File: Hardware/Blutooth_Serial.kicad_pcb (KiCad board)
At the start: 2 copper layers, 67.4 x 48.5 mm, 22 parts, among them J2 Conn_01x04_Pin, U2 MAX3232, U3 LM2596S-5

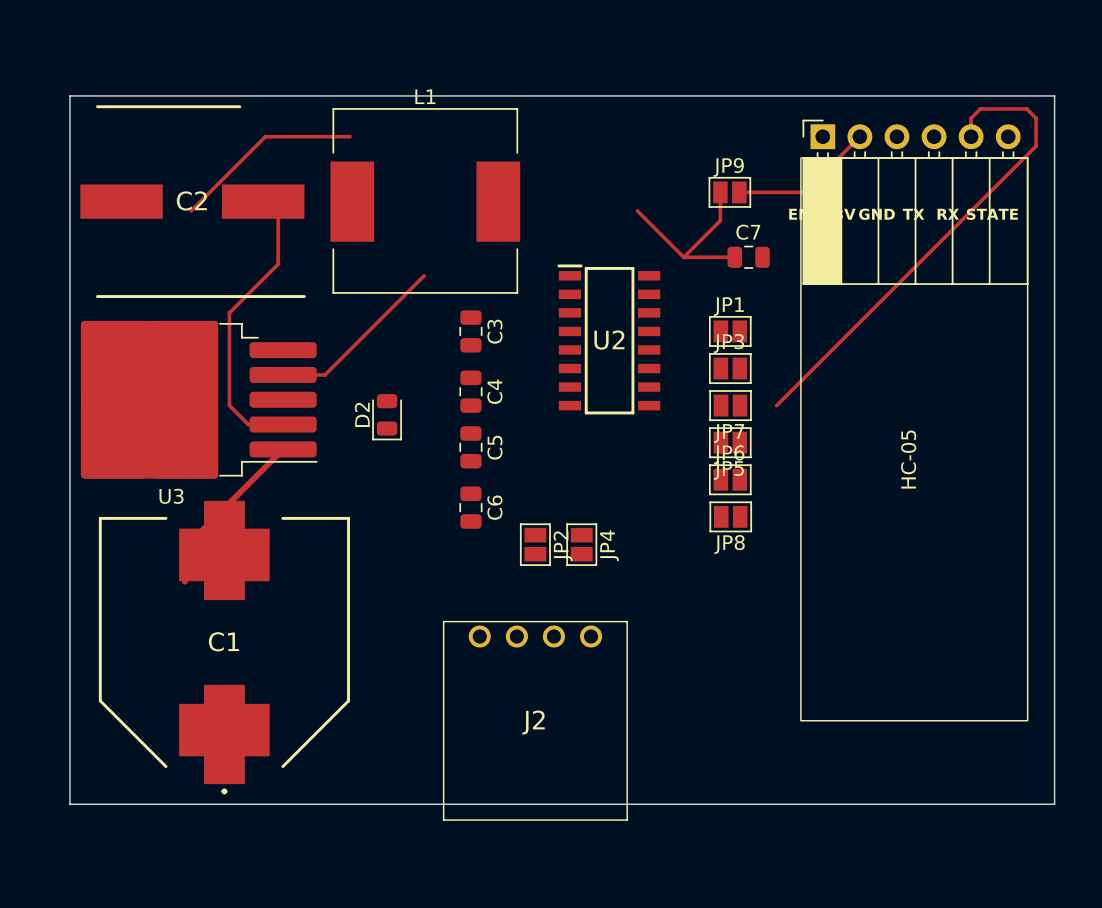
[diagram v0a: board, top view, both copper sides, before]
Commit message: changes
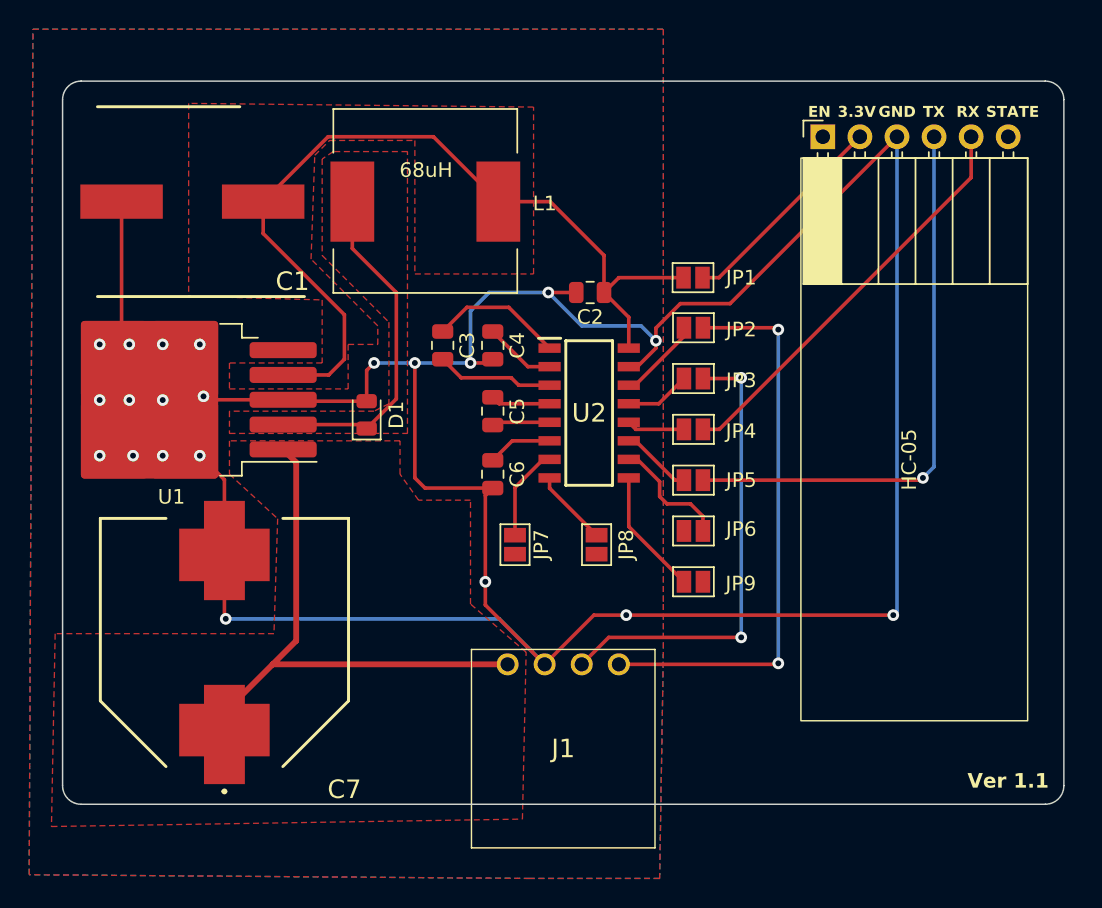
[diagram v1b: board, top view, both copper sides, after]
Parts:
- added G***: LOGO, Library:LOGO, B.Cu at (108.7, 109.0)
- C1: renamed from C2; footprint my_lib:220uF_SMD_CAP -> Library:220uF_SMD_CAP
- C2: renamed from C7; footprint Capacitor_SMD:C_0805_2012Metric -> Library:C_0805_2012Metric
- C3, C4, C5, C6: footprint Capacitor_SMD:C_0805_2012Metric -> Library:C_0805_2012Metric
- C7: renamed from C1; footprint my_lib:470uF_SMD_CAP -> Library:470uF_SMD_CAP
- D1: renamed from D2; footprint Diode_SMD:D_0805_2012Metric -> Library:D_0805_2012Metric
- IC1: footprint my_lib:HC-05 -> Library:HC-05
- J1: renamed from J2; footprint my_lib:male_pin_4 -> Library:male_pin_4
- JP1: renamed from JP9; footprint Jumper:SolderJumper-2_P1.3mm_Open_Pad1.0x1.5mm -> Library:SolderJumper-2_P1.3mm_Open_Pad1.0x1.5mm
- JP2: renamed from JP1; footprint Jumper:SolderJumper-2_P1.3mm_Open_Pad1.0x1.5mm -> Library:SolderJumper-2_P1.3mm_Open_Pad1.0x1.5mm
- JP3, JP5, JP6: footprint Jumper:SolderJumper-2_P1.3mm_Open_Pad1.0x1.5mm -> Library:SolderJumper-2_P1.3mm_Open_Pad1.0x1.5mm
- JP4: renamed from JP7; footprint Jumper:SolderJumper-2_P1.3mm_Open_Pad1.0x1.5mm -> Library:SolderJumper-2_P1.3mm_Open_Pad1.0x1.5mm
- JP7: renamed from JP2; footprint Jumper:SolderJumper-2_P1.3mm_Open_Pad1.0x1.5mm -> Library:SolderJumper-2_P1.3mm_Open_Pad1.0x1.5mm
- JP8: renamed from JP4; footprint Jumper:SolderJumper-2_P1.3mm_Open_Pad1.0x1.5mm -> Library:SolderJumper-2_P1.3mm_Open_Pad1.0x1.5mm
- JP9: renamed from JP8; footprint Jumper:SolderJumper-2_P1.3mm_Open_Pad1.0x1.5mm -> Library:SolderJumper-2_P1.3mm_Open_Pad1.0x1.5mm
- L1: footprint my_lib:L_12x12mm_H6mm -> Library:L_12x12mm_H6mm
- U1: renamed from U3; footprint Package_TO_SOT_SMD:TO-263-5_TabPin3 -> Library:TO-263-5_TabPin3
- U2: footprint my_lib:MAX3232EIDR -> Library:MAX3232EIDR
- moved C2 11.1 mm to (80.6, 76.7), turned to 180 degrees
- moved JP1 6.36 mm to (87.6, 75.7)
- moved U2 5.15 mm to (80.5, 85.0)
- moved JP9 5.13 mm to (87.7, 96.5)
- moved JP6 4.32 mm to (87.7, 93.0)
- moved JP5 3.60 mm to (87.7, 89.6)
- moved C4 3.51 mm to (73.9, 80.3)
- moved JP4 3.02 mm to (87.7, 86.1)
- moved C5 2.89 mm to (73.9, 84.8)
- moved C6 2.73 mm to (73.9, 89.2)
- moved J1 2.69 mm to (78.7, 108.0)
- moved JP3 2.62 mm to (87.7, 82.6)
- moved JP2 2.54 mm to (87.7, 79.1)
- moved C3 2.16 mm to (70.5, 80.3)
- moved D1 1.40 mm to (65.3, 85.1)
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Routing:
- net GND: track 0.00 -> 205.8 mm, vias 0 -> 21
- net Net-(J1-Pin_4): track 0.00 -> 39.0 mm, vias 0 -> 2
- net T1IN: track 0.00 -> 38.8 mm, vias 0 -> 1
- net Net-(J1-Pin_3): track 0.00 -> 32.1 mm, vias 0 -> 2
- net +24V: track 11.9 -> 38.0 mm
- net 5V: track 39.4 -> 59.2 mm
- net Net-(U2-C1+): track 0.00 -> 9.16 mm
- net Net-(JP9-B): track 0.00 -> 8.68 mm
- net Net-(JP6-B): track 0.00 -> 8.29 mm
- net Net-(U2-C1-): track 0.00 -> 8.06 mm
- net Net-(JP7-A): track 0.00 -> 6.43 mm
- net Net-(JP2-A): track 0.00 -> 5.76 mm
- net Net-(JP8-A): track 0.00 -> 5.26 mm
- net R1OUT: track 33.3 -> 28.3 mm
- net Net-(IC1-Vcc): track 9.83 -> 14.8 mm
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- added copper zone on F.Cu, net +24V
- added copper zone on F.Cu, net 5V
- added copper zone on B.Cu, net GND
- added copper zone on F.Cu, net GND
- added copper zone on F.Cu, net Net-(D1-K)
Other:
- board size 67.4 x 48.5 mm -> 68.6 x 49.5 mm
- board text added: "Ver 1.1"
